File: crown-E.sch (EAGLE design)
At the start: 97 parts

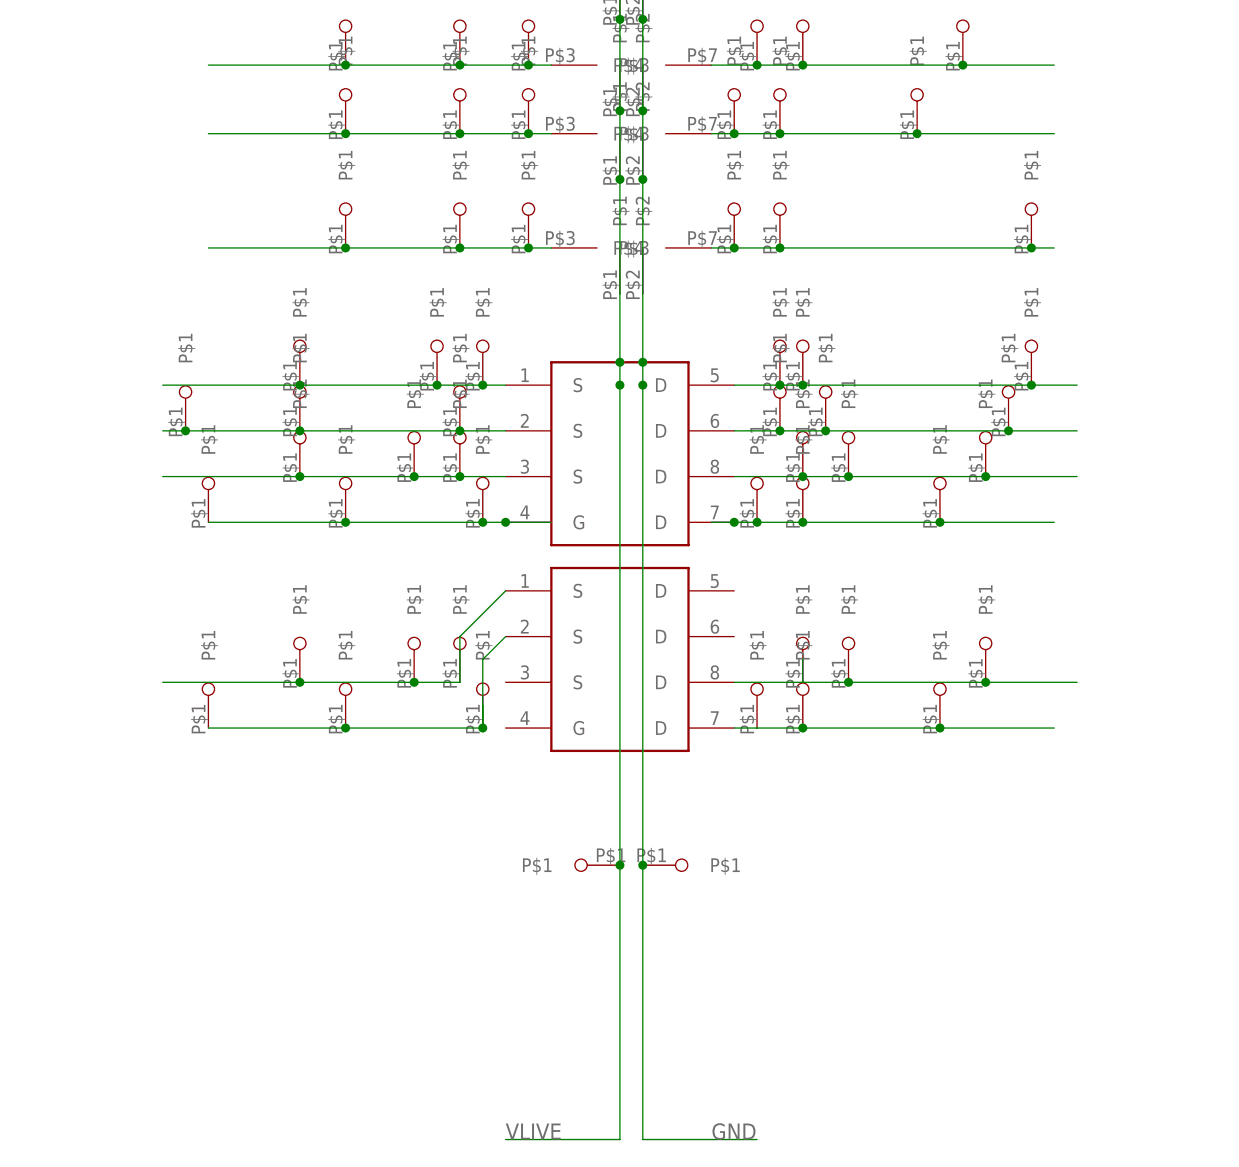
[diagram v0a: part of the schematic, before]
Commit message: Added final panel! whooo!
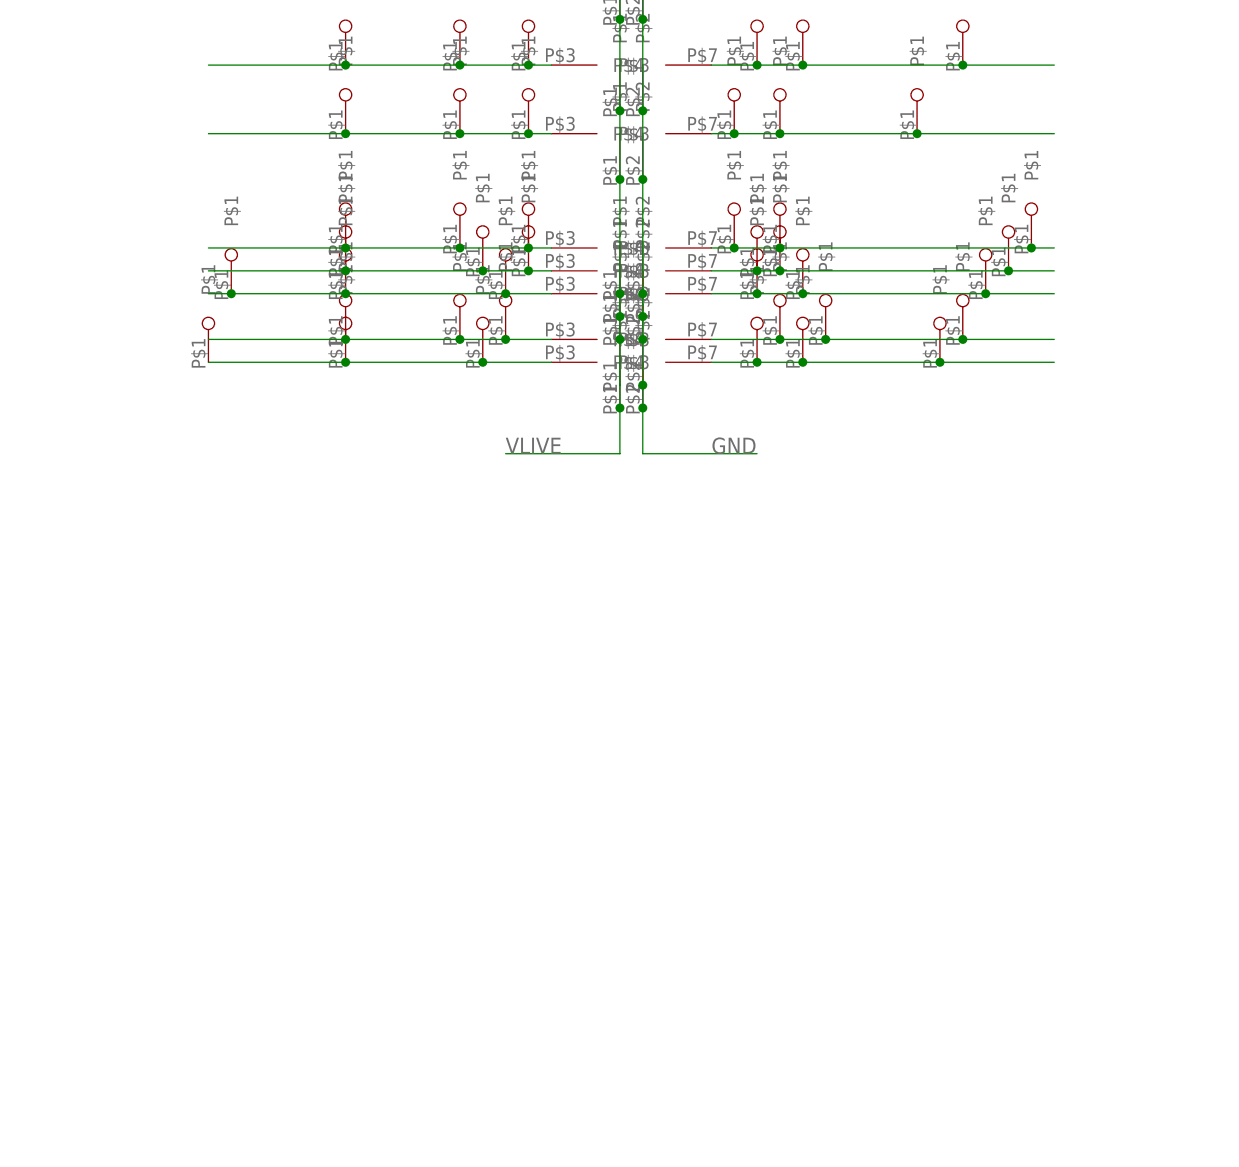
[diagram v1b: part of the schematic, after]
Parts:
- removed U$72, U$81: NDS8434, SparkFun-DiscreteSemi:NDS8434
- removed U$73, U$74, U$75, U$76, U$77, U$78, U$79, U$80, U$82, U$83: SMD_PAD, pcb_crown:SMD_PAD
- U$1, U$3, U$8, U$9: value SMD_PAD -> SMD_BREADBOARD; device pcb_crown:SMD_PAD -> pcb_crown:SMD_BREADBOARD
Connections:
- removed net N$23: U$1.P$1, U$3.P$1, U$77.P$1, U$81.S@1
- removed net N$24: U$75.P$1, U$76.P$1, U$80.P$1, U$81.D@2
- removed net N$25: U$73.P$1, U$74.P$1, U$79.P$1, U$81.D@1
- removed net N$26: U$78.P$1, U$8.P$1, U$81.S@2, U$9.P$1
- net GND: now also U$1.P$2, U$3.P$2, U$8.P$2, U$9.P$2; no longer U$83.P$1
- net N$18: now also U$8.P$4; no longer U$72.D@4
- net N$19: now also U$9.P$4; no longer U$72.D@3
- net N$2: now also U$1.P$3; no longer U$72.G
- net N$20: now also U$3.P$4; no longer U$72.D@2
- net N$21: now also U$1.P$4; no longer U$72.D@1
- net N$6: now also U$3.P$3; no longer U$72.S@3
- net N$7: now also U$9.P$3; no longer U$72.S@2
- net N$8: now also U$8.P$3; no longer U$72.S@1
- net VLIVE: now also U$1.P$1, U$3.P$1, U$8.P$1, U$9.P$1; no longer U$82.P$1
